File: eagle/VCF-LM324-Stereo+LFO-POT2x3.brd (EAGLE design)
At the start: 55.9 x 61 mm, 50 parts, among them IC1 LM324, J1 CONN-3P-3P, J2 CONN-3P-3P, J3 CONN-2P2P/H

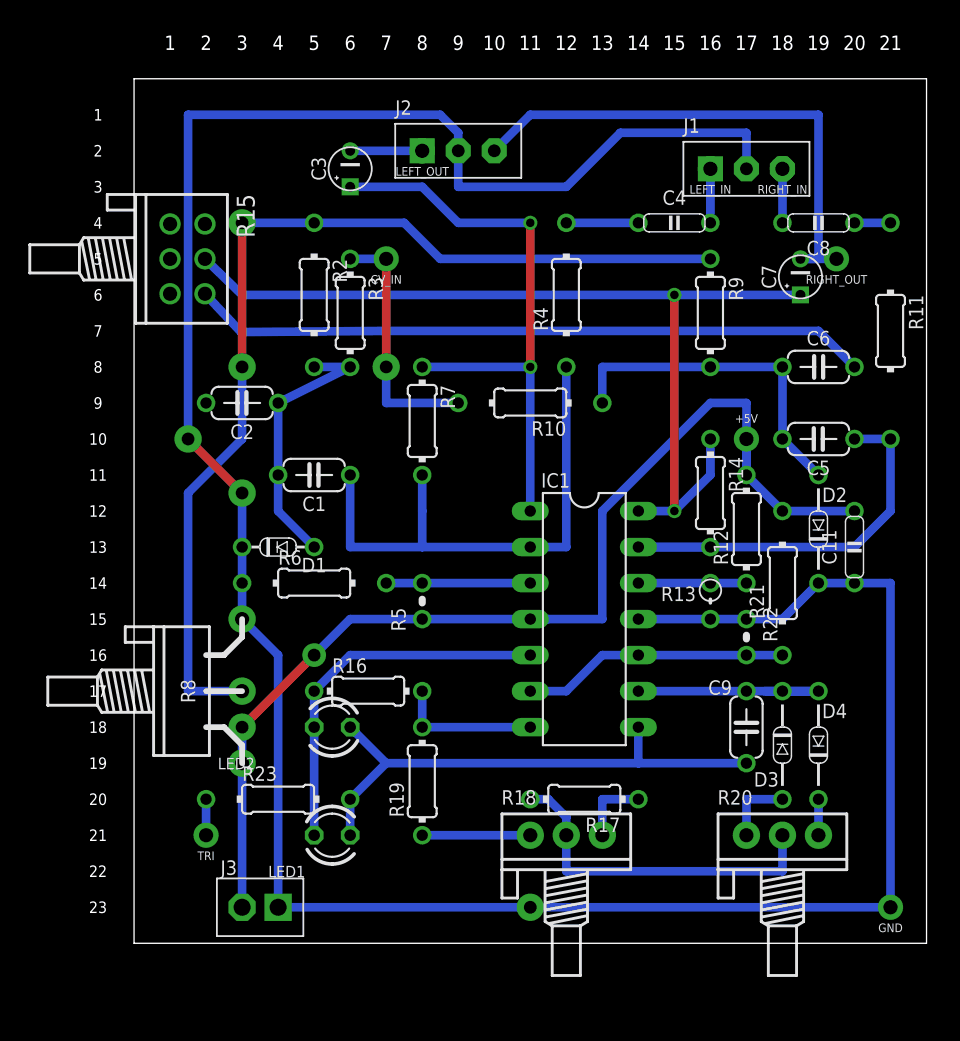
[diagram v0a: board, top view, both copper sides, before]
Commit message: ...
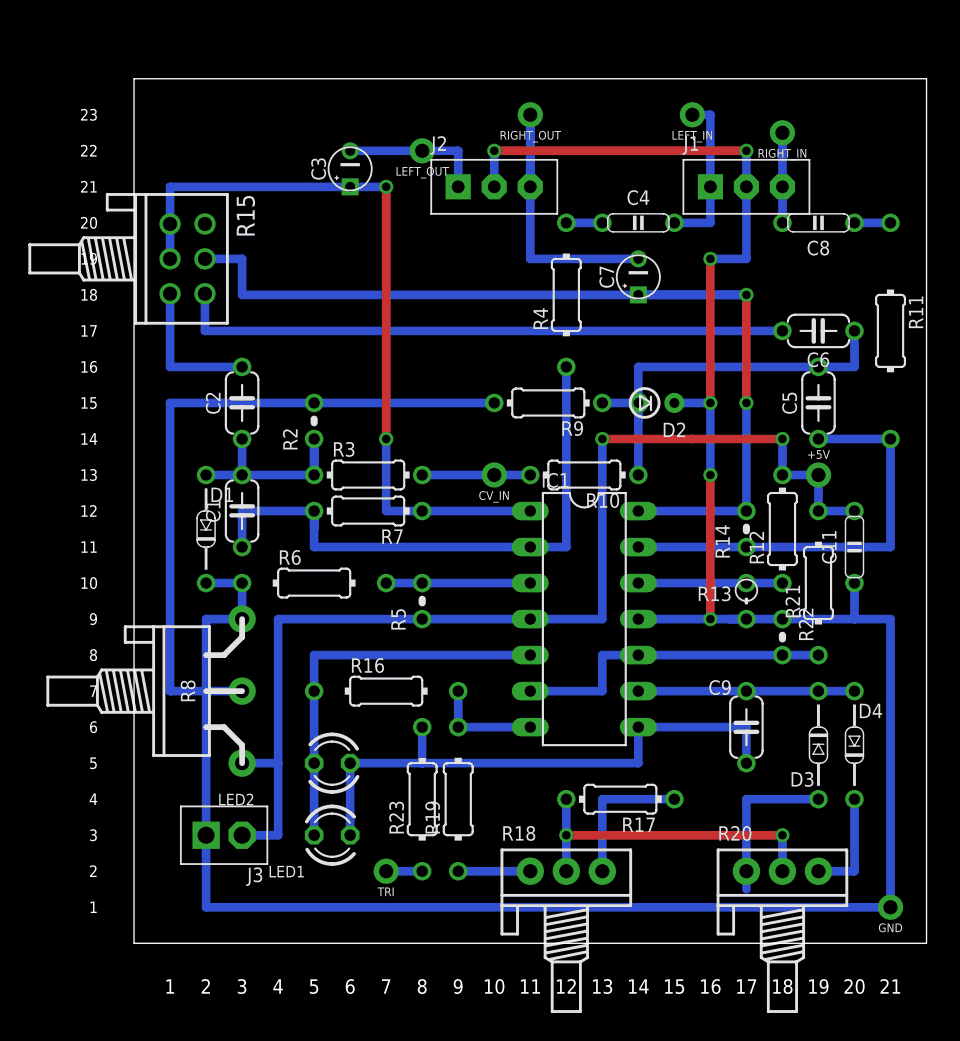
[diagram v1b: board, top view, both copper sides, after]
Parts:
- D1: device d:DO34-5 -> d:DO34-7V
- D2: device d:DO34-7V -> d:DO35-2_54
- R10: device r:0204/10 -> r:0204/7
- R14: device r:0204/7-V -> r:0204V
- R16: device r:0204/7 -> r:0204/10
- R19: device r:0204/7-V -> r:0204/10-V
- R2: device r:0204/10-V -> r:0204V
- R3, R9: device r:0204/7-V -> r:0204/7
- moved RIGHT_OUT 23.9 mm to (30.5, 58.4)
- moved CV_IN 17.0 mm to (27.9, 33.0)
- moved D2 14.5 mm to (39.4, 38.1), turned to 180 degrees
- moved R9 13.1 mm to (31.8, 38.1)
- moved TRI 13.0 mm to (20.3, 5.08)
- moved R3 11.5 mm to (19.1, 33.0), turned to 0 degrees
- moved C7 11.4 mm to (38.1, 47.0)
- moved R23 10.2 mm to (22.9, 10.2), turned to 90 degrees
- moved R2 8.89 mm to (15.2, 36.8), turned to 90 degrees
- moved R7 7.41 mm to (19.1, 30.5), turned to 90 degrees
- moved J3 7.18 mm to (7.62, 7.62), turned to 180 degrees
- moved R10 6.35 mm to (34.3, 33.0)
- moved C1 5.68 mm to (10.2, 30.5), turned to 90 degrees
- moved +5V 5.68 mm to (50.8, 33.0)
- moved D1 5.24 mm to (7.62, 29.2)
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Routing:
- net N$5: track 72.5 -> 48.3 mm, vias 2 -> 0
- net RIGHT_OUT: track 37.9 -> 22.9 mm
- net GND: track 191.2 -> 176.5 mm, vias 3 -> 6
- net N$4: track 41.7 -> 53.3 mm
- net N$8: track 18.1 -> 7.62 mm, vias 1 -> 0
- net N$3: track 0.00 -> 10.2 mm
- net LEFT_IN: track 3.81 -> 11.4 mm
- net TRIM_1_A: track 5.08 -> 11.4 mm
- net N$16: track 23.9 -> 29.2 mm
- net TRIM_1_B: track 2.54 -> 7.62 mm
- net TRIM_2_A: track 5.08 -> 10.2 mm
- net LEFT_OUT: track 5.08 -> 10.2 mm
- net N$11: track 48.0 -> 43.3 mm
- net N$12: track 66.9 -> 71.2 mm, vias 3 -> 2
- net N$9: track 19.4 -> 15.2 mm
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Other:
- board text removed: "Cutoff"
- board text removed: "RES"

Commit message: ...
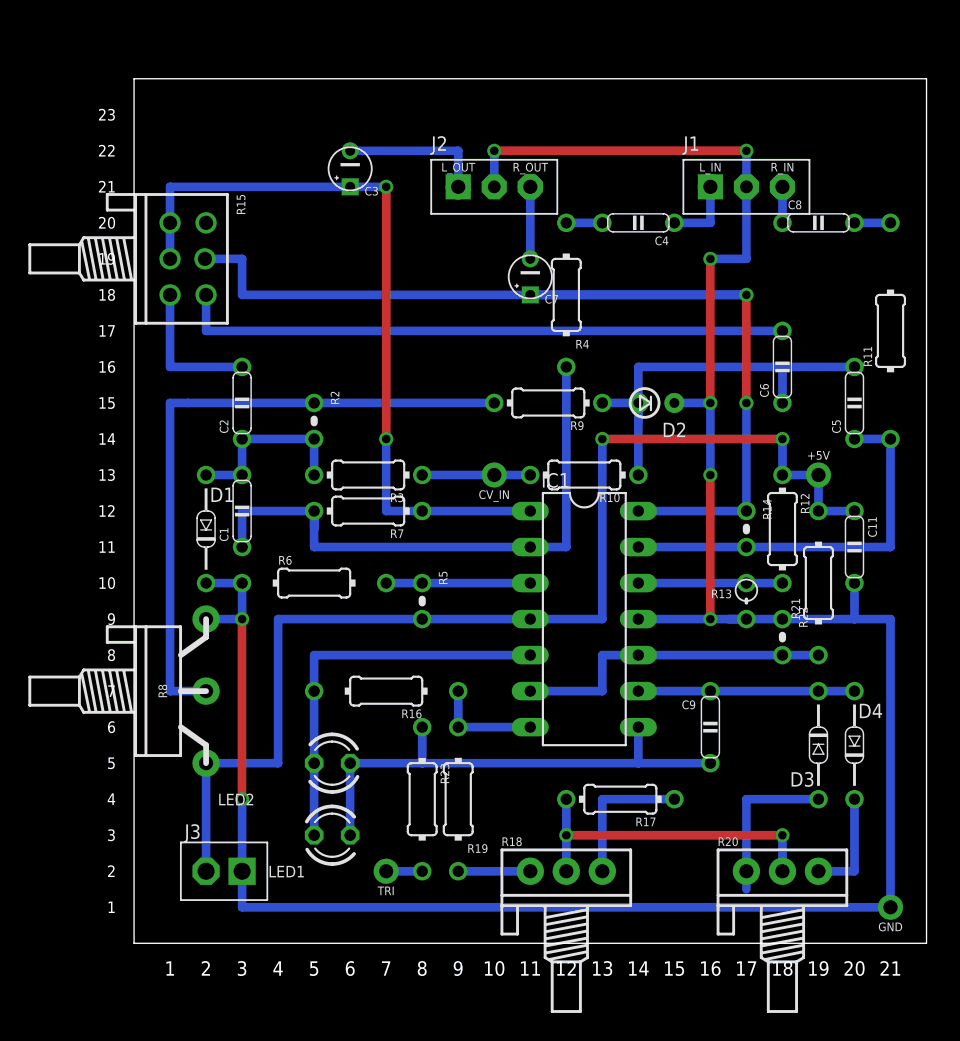
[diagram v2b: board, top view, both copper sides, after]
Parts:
- removed LEFT_IN, RIGHT_IN: AUDIO_IN, pad:SPAD
- removed LEFT_OUT, RIGHT_OUT: AUDIO_OUT, pad:SPAD
- added L_IN, R_IN: AUDIO_IN, pad:SPAD
- added L_OUT, R_OUT: AUDIO_OUT, pad:SPAD
- C1, C2: value 100nF -> 0.1uF; device c:C050-024X044 -> c:C050-020X044
- C3, C7: device c:E2,5-3 -> c:E2,5-3/V
- C5, C6: device c:C050-024X044 -> c:C050-020X044
- C9: device c:C050-024X044/V -> c:C050-020X044/V
- J1: value CONN-3P-3P -> A_IN
- J2: value CONN-3P-3P -> A_OUT
- R15: value POT-STEREO -> 10k
- R8: value POT-P5 -> (none)
- moved C7 7.62 mm to (30.5, 47.0)
- moved J3 3.59 mm to (10.2, 5.08), turned to 0 degrees
- moved C6 3.59 mm to (48.3, 40.6), turned to 90 degrees
- moved C5 2.54 mm to (53.3, 38.1)
- moved C9 2.54 mm to (43.2, 15.2)
- moved R8 1.27 mm to (5.08, 17.8)
- turned C11 to 270 degrees
- turned C4 to 180 degrees
- turned C8 to 0 degrees
- turned R11 to 90 degrees
- turned R12 to 180 degrees
- turned R14 to 270 degrees
- turned R16 to 180 degrees
- turned R19 to 180 degrees
- turned R2 to 270 degrees
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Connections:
- net LEFT_IN: now also L_IN.1; no longer LEFT_IN.1
- net LEFT_OUT: now also L_OUT.1; no longer LEFT_OUT.1
- net N$10: now also R4.2; no longer R4.1
- net N$12: now also R14.1; no longer R14.2
- net N$13: now also R12.1; no longer R12.2
- net N$14: now also R16.1, R19.2; no longer R16.2, R19.1
- net N$15: now also R16.2; no longer R16.1
- net N$17: now also R11.1, R14.2; no longer R11.2, R14.1
- net N$2: now also R4.1; no longer R4.2
- net N$20: now also R11.2; no longer R11.1
- net N$28: now also R23.1; no longer R23.2
- net N$5: now also R2.1; no longer R2.2
- net N$7: now also R5.1; no longer R5.2
- net N$8: now also R3.1; no longer R3.2
- net N$9: now also R2.2, R3.2; no longer R2.1, R3.1
- net RIGHT_IN: now also R_IN.1; no longer RIGHT_IN.1
- net RIGHT_OUT: now also R_OUT.1; no longer RIGHT_OUT.1
- net TRIM_2_B: now also R19.1; no longer R19.2
- net TRI_OUT: now also R23.2; no longer R23.1
- net VCC: now also R12.2, R5.2; no longer R12.1, R5.1
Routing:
- net RIGHT_OUT: track 22.9 -> 5.08 mm
- net N$12: track 71.2 -> 78.8 mm
- net LEFT_IN: track 11.4 -> 5.08 mm
- net N$28: track 40.6 -> 35.6 mm
- net RIGHT_IN: track 6.35 -> 2.54 mm
- net GND: track 176.5 -> 174.0 mm, vias 6 -> 8
- net N$5: track 48.3 -> 45.7 mm
- net N$17: track 30.5 -> 27.9 mm
- net N$9: track 15.2 -> 12.7 mm
- net VCC: track 78.7 -> 81.3 mm
